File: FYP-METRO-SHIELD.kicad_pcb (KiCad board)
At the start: 2 copper layers, 68.6 x 53.3 mm, 40 parts, among them J1 Power, J2 Digital/PWM, J3 Analog, J4 Digital/PWM, J5 Conn_01x08, Q2 NPN, U1 MCP602, U2 LM393, U3 LM386

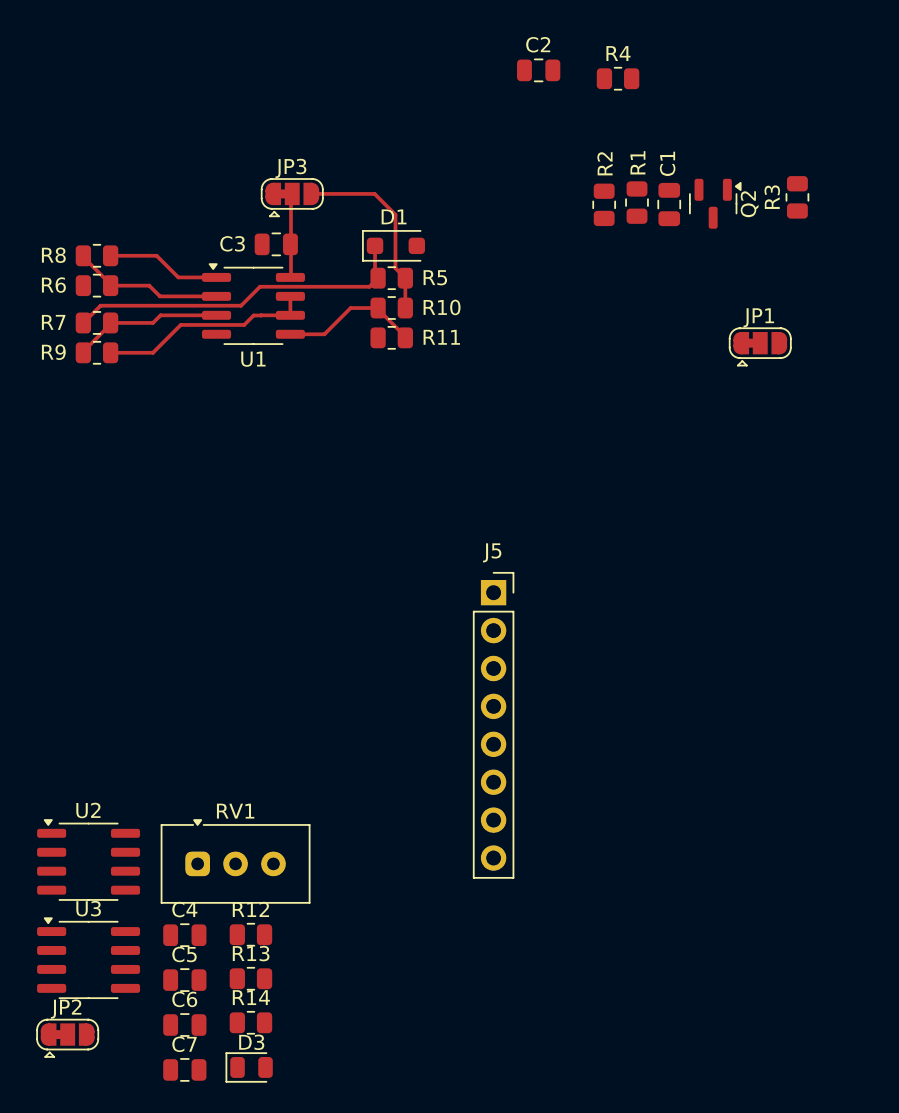
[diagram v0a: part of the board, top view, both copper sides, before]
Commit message: aaa
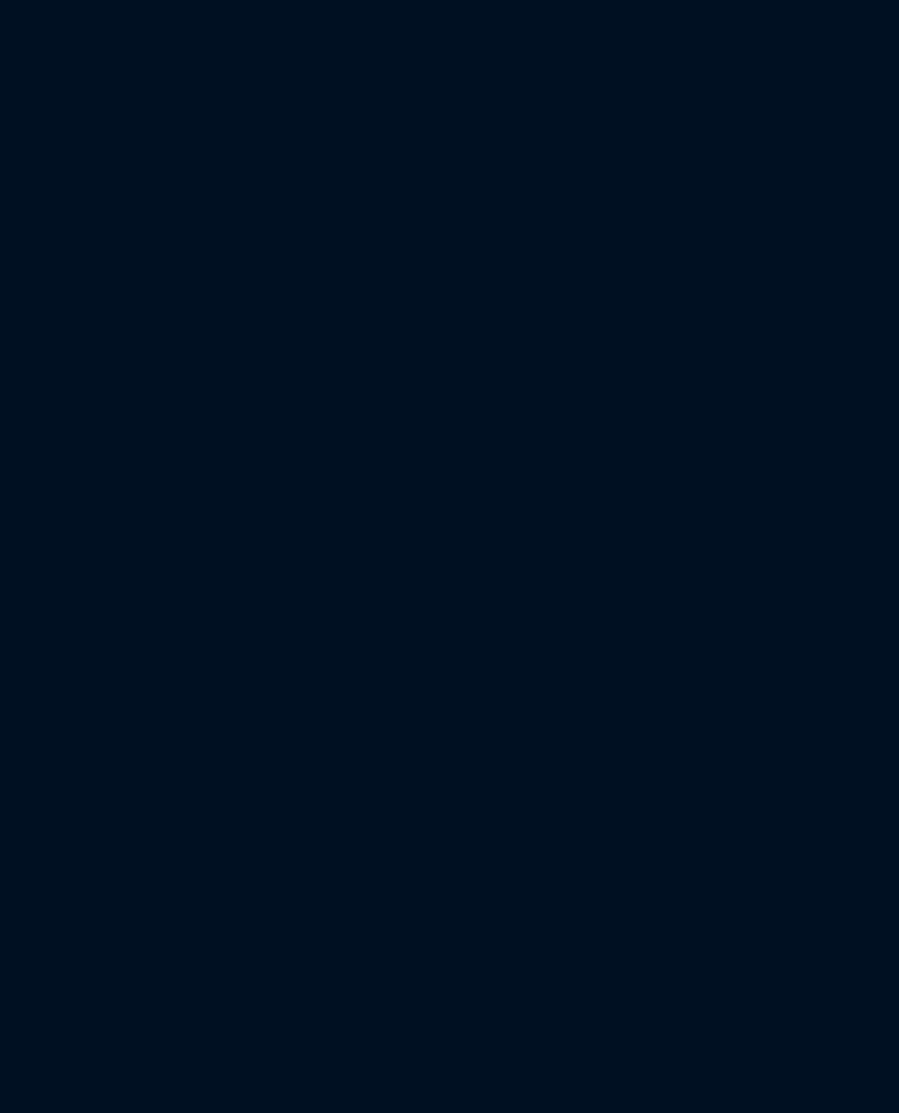
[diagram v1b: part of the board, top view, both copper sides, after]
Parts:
- removed C1, C2: 0.1u, Capacitor_SMD:C_0805_2012Metric
- removed C3, C4, C5, C6: 100n, Capacitor_SMD:C_0805_2012Metric
- removed C7: 47n, Capacitor_SMD:C_0805_2012Metric
- removed D1: 2V, Diode_SMD:D_SOD-123F
- removed D3: LED, LED_SMD:LED_0805_2012Metric
- removed J5: Conn_01x08, Connector_PinSocket_2.54mm:PinSocket_1x08_P2.54mm_Vertical
- removed JP1, JP2, JP3: Jumper_3_Bridged12, Jumper:SolderJumper-3_P1.3mm_Bridged12_RoundedPad1.0x1.5mm
- removed Q2: NPN, Package_TO_SOT_SMD:SOT-23
- removed R1, R4, R6, R7: 10k, Resistor_SMD:R_0805_2012Metric
- removed R10: 9.1k, Resistor_SMD:R_0805_2012Metric
- removed R11: 1k, Resistor_SMD:R_0805_2012Metric
- removed R12, R13: 1.4k, Resistor_SMD:R_0805_2012Metric
- removed R14: 220, Resistor_SMD:R_0805_2012Metric
- removed R2: 680k, Resistor_SMD:R_0805_2012Metric
- removed R3: 4.3k, Resistor_SMD:R_0805_2012Metric
- removed R5: 4k, Resistor_SMD:R_0805_2012Metric
- removed R8, R9: 1M, Resistor_SMD:R_0805_2012Metric
- removed RV1: 100k, Potentiometer_THT:Potentiometer_Vishay_T93YA_Vertical
- removed U1: MCP602, Package_SO:SOIC-8_3.9x4.9mm_P1.27mm
- removed U2: LM393, Package_SO:SOIC-8_3.9x4.9mm_P1.27mm
- removed U3: LM386, Package_SO:SOIC-8_3.9x4.9mm_P1.27mm
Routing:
- net Net-(D1-K): track 23.2 -> 0.00 mm
- net /A2: track 14.4 -> 0.00 mm
- net +5V: track 12.7 -> 0.00 mm
- net Net-(U1A--): track 10.3 -> 0.00 mm
- net Net-(U1A-+): track 10.1 -> 0.00 mm
- net Net-(U1B-+): track 9.38 -> 0.00 mm
- net /A1: track 7.70 -> 0.00 mm
- net Net-(JP3-C): track 5.65 -> 0.00 mm

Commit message: LOL
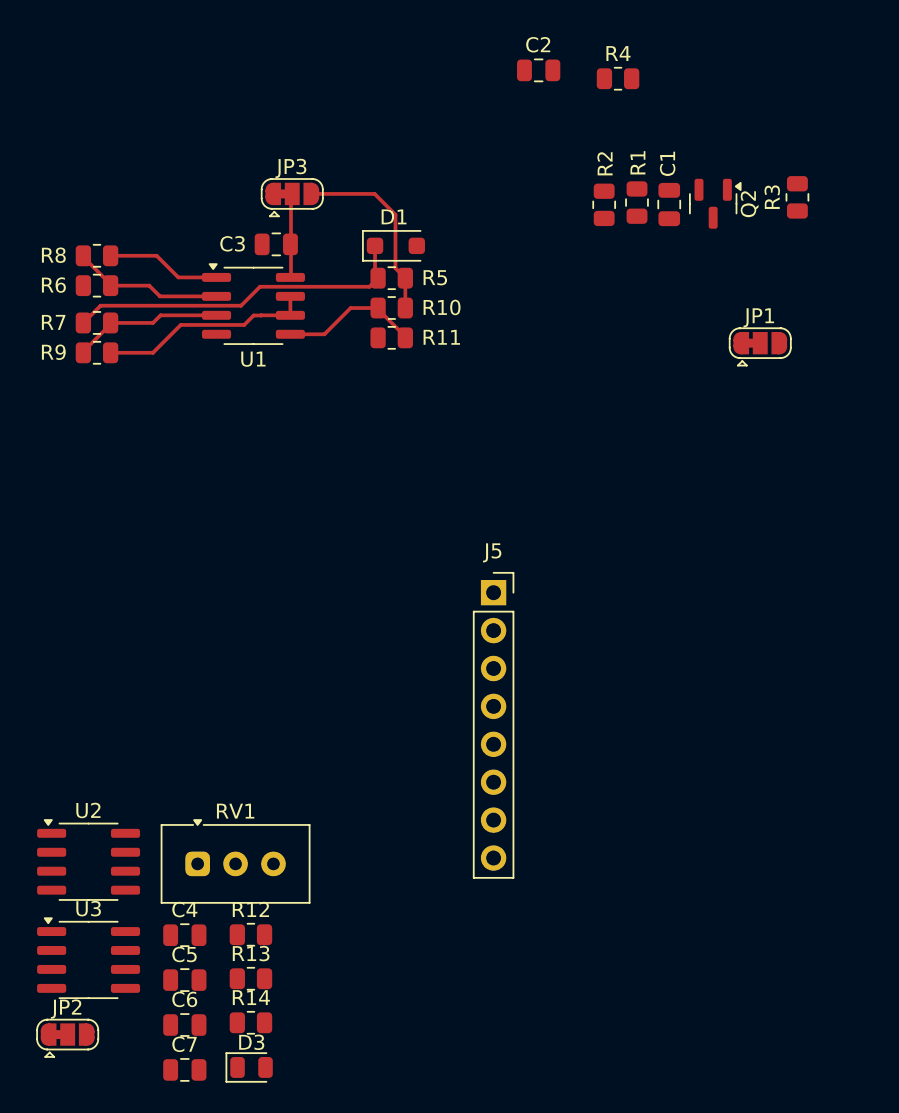
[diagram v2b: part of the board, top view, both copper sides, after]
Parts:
- added C1: 0.1u, Capacitor_SMD:C_0805_2012Metric, F.Cu at (60.1, 46.8)
- added C2: 0.1u, Capacitor_SMD:C_0805_2012Metric, F.Cu at (51.3, 37.8)
- added C3: 100n, Capacitor_SMD:C_0805_2012Metric, F.Cu at (33.8, 49.5)
- added C4: 100n, Capacitor_SMD:C_0805_2012Metric, F.Cu at (27.6, 95.8)
- added C5: 100n, Capacitor_SMD:C_0805_2012Metric, F.Cu at (27.6, 98.8)
- added C6: 100n, Capacitor_SMD:C_0805_2012Metric, F.Cu at (27.6, 101.8)
- added C7: 47n, Capacitor_SMD:C_0805_2012Metric, F.Cu at (27.6, 104.8)
- added D1: 2V, Diode_SMD:D_SOD-123F, F.Cu at (41.8, 49.6)
- added D3: LED, LED_SMD:LED_0805_2012Metric, F.Cu at (32.1, 104.6)
- added J5: Conn_01x08, Connector_PinSocket_2.54mm:PinSocket_1x08_P2.54mm_Vertical, F.Cu at (48.3, 72.8)
- added JP1: Jumper_3_Bridged12, Jumper:SolderJumper-3_P1.3mm_Bridged12_RoundedPad1.0x1.5mm, F.Cu at (66.2, 56.1)
- added JP2: Jumper_3_Bridged12, Jumper:SolderJumper-3_P1.3mm_Bridged12_RoundedPad1.0x1.5mm, F.Cu at (19.8, 102.4)
- added JP3: Jumper_3_Bridged12, Jumper:SolderJumper-3_P1.3mm_Bridged12_RoundedPad1.0x1.5mm, F.Cu at (34.8, 46.1)
- added Q2: NPN, Package_TO_SOT_SMD:SOT-23, F.Cu at (63.0, 46.8)
- added R1: 10k, Resistor_SMD:R_0805_2012Metric, F.Cu at (57.9, 46.7)
- added R10: 9.1k, Resistor_SMD:R_0805_2012Metric, F.Cu at (41.5, 53.8)
- added R11: 1k, Resistor_SMD:R_0805_2012Metric, F.Cu at (41.5, 55.8)
- added R12: 1.4k, Resistor_SMD:R_0805_2012Metric, F.Cu at (32.1, 95.7)
- added R13: 1.4k, Resistor_SMD:R_0805_2012Metric, F.Cu at (32.1, 98.7)
- added R14: 220, Resistor_SMD:R_0805_2012Metric, F.Cu at (32.1, 101.6)
- added R2: 680k, Resistor_SMD:R_0805_2012Metric, F.Cu at (55.7, 46.8)
- added R3: 4.3k, Resistor_SMD:R_0805_2012Metric, F.Cu at (68.7, 46.3)
- added R4: 10k, Resistor_SMD:R_0805_2012Metric, F.Cu at (56.7, 38.4)
- added R5: 4k, Resistor_SMD:R_0805_2012Metric, F.Cu at (41.5, 51.8)
- added R6: 10k, Resistor_SMD:R_0805_2012Metric, F.Cu at (21.8, 52.2)
- added R7: 10k, Resistor_SMD:R_0805_2012Metric, F.Cu at (21.8, 54.8)
- added R8: 1M, Resistor_SMD:R_0805_2012Metric, F.Cu at (21.8, 50.2)
- added R9: 1M, Resistor_SMD:R_0805_2012Metric, F.Cu at (21.8, 56.8)
- added RV1: 100k, Potentiometer_THT:Potentiometer_Vishay_T93YA_Vertical, F.Cu at (28.5, 91.0)
- added U1: MCP602, Package_SO:SOIC-8_3.9x4.9mm_P1.27mm, F.Cu at (32.2, 53.6)
- added U2: LM393, Package_SO:SOIC-8_3.9x4.9mm_P1.27mm, F.Cu at (21.2, 90.9)
- added U3: LM386, Package_SO:SOIC-8_3.9x4.9mm_P1.27mm, F.Cu at (21.2, 97.4)
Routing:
- net Net-(D1-K): track 0.00 -> 23.2 mm
- net /A2: track 0.00 -> 14.4 mm
- net +5V: track 0.00 -> 12.7 mm
- net Net-(U1A--): track 0.00 -> 10.3 mm
- net Net-(U1A-+): track 0.00 -> 10.1 mm
- net Net-(U1B-+): track 0.00 -> 9.38 mm
- net /A1: track 0.00 -> 7.70 mm
- net Net-(JP3-C): track 0.00 -> 5.65 mm
